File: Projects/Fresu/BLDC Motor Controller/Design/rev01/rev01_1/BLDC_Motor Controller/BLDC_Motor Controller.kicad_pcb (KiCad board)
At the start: 4 copper layers, 100 x 75 mm, 178 parts, among them CN1 XT60PW-M, J1 Conn_01x08, J2 Conn_01x06, J3 Conn_01x03, J4 7461084, J5 7461084, J6 7461084, J7 Conn_01x06, J8 XH-2PWBPZ, J9 TYPE-C-31-M-12, Q1 HSBA15810C, Q2 HSBA15810C, Q3 HSBA15810C, Q4 HSBA15810C, Q5 HSBA15810C, Q6 HSBA15810C, SW1 PTS526SK15SMTR2LFS, U1 STM32F405RGTx, U2 DRV8302_DCA_56, U3 S4B-XH-SM4-TB-(LF)(SN), U4 SN65HVD230, U5 AMS1117-3.3, U6 PUSB3AB6Z, Y1 8MHz

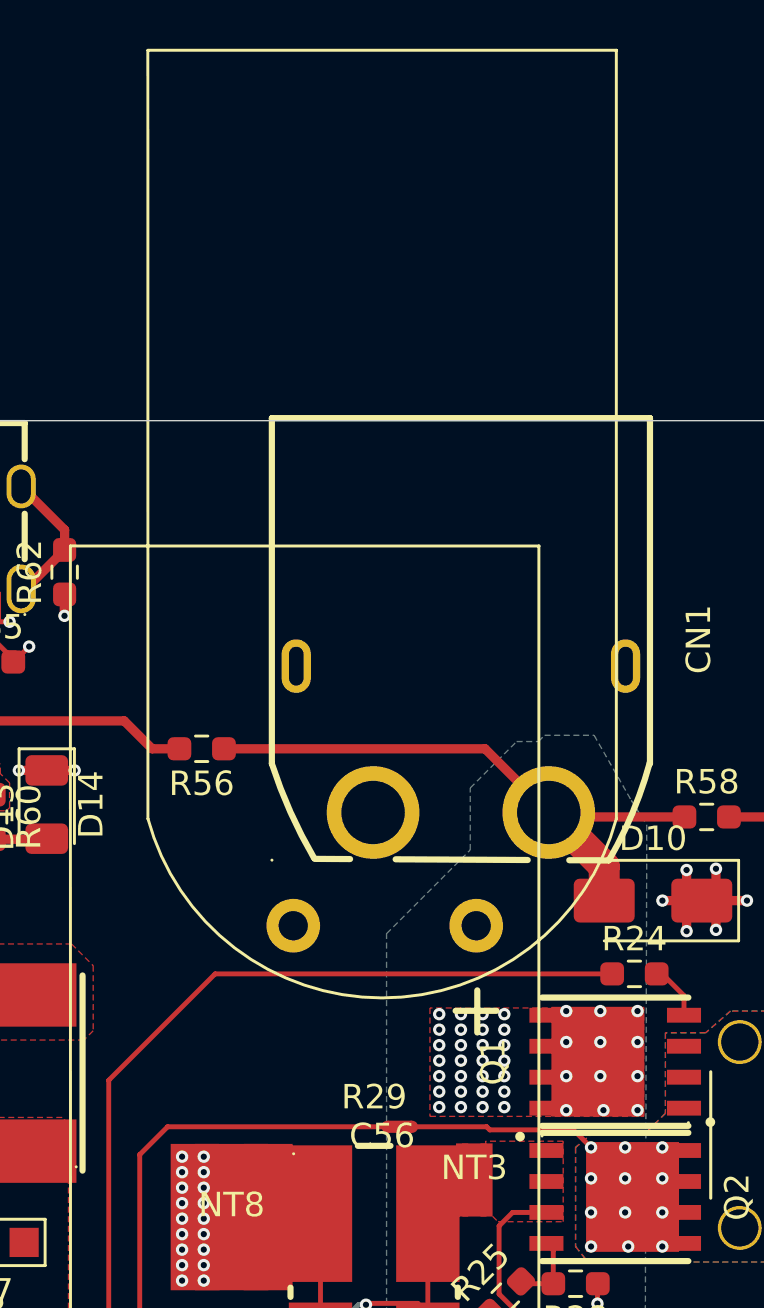
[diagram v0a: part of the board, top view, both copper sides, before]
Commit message: Update 22
Continued DRC
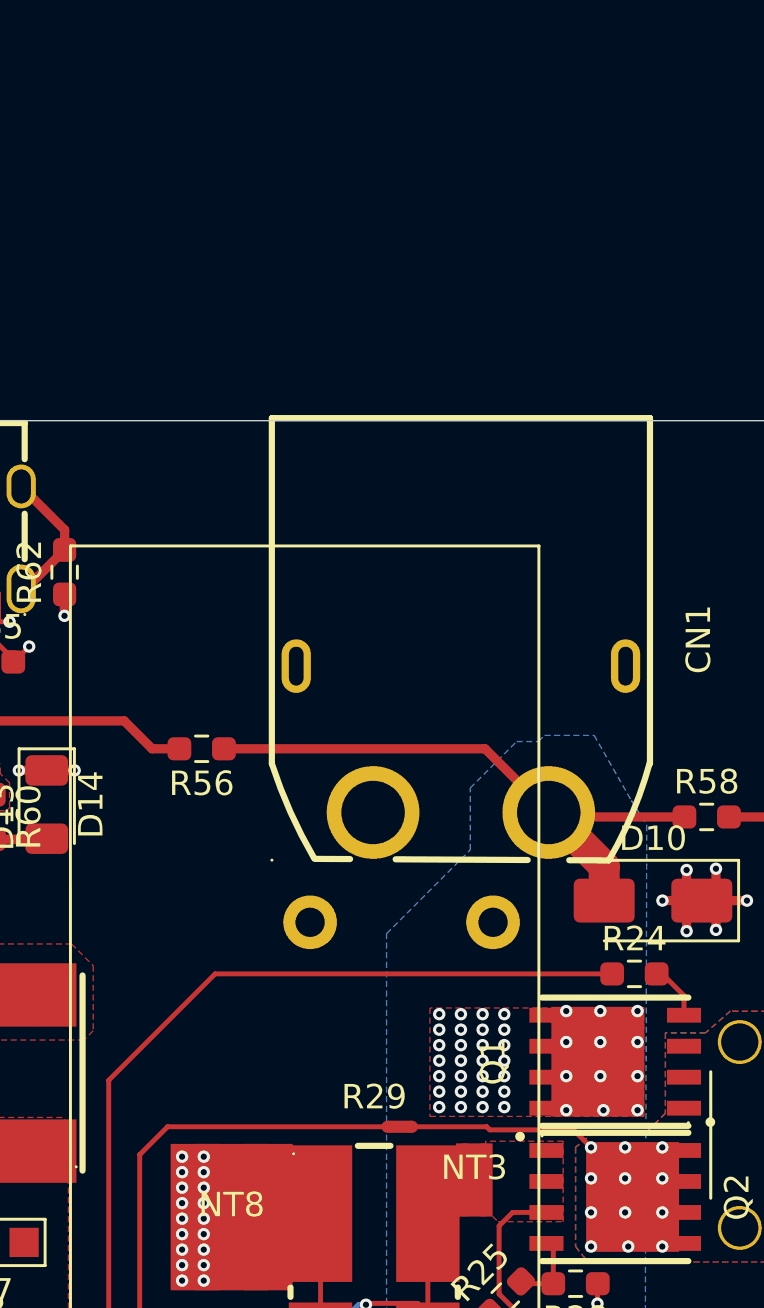
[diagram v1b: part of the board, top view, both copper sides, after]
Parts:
- C56: moved to B.Cu
- moved C56 0.78 mm to (238.6, 119.6)
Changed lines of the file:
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@@
     (pad "2" thru_hole circle locked (at 5.643701 0.113589 180) (size 2.2 2.2) (drill 1.2) (layers "*.Cu" "*.Mask")
       (net 2 "GND") (pinfunction "2") (pintype "passive"))
-    (model "C:/Users/Will/Downloads/Libraries (1)/Libraries/3D Models/CAP_LAT_SIDE.step"
+    (model "C:/Users/Will/Downloads/Libraries (1)/Libraries/3D Models/CAP_LAT_SIDE.step" hide
       (offset (xyz 1.9 -5.1 9.5))
       (scale (xyz 2.5 2.5 2.5))
@@
       (net 62 "H3_LOW") (pinfunction "2") (pintype "passive"))
   )
-  (footprint "DF_ESC_Footprint_Library:CAP-TH_BD18.0-P7.50-D1.2-SIDE" (layer "F.Cu")
-    (at 237.871 120.015 180)
-    (descr "CAP-TH_BD18.0-P7.50-D1.2-FD footprint")
-    (tags "CAP-TH_BD18.0-P7.50-D1.2-FD footprint")
-    (property "Capacitance" "820uF")
-    (property "LCSC" "C443097")
-    (property "Sheetfile" "INPUT PROTECTION.kicad_sch")
-    (property "Sheetname" "INPUT PROTECTION")
-    (property "ki_keywords" "C443097")
-    (attr through_hole)
-    (fp_text reference "C56" (at 2 -8.5) (layer "F.SilkS")
-        (effects (font (size 1 1) (thickness 0.15)))
-    )
-    (fp_text value "LKMI2501K821MF" (at 0 2.863602) (layer "F.Fab")
-        (effects (font (size 1 1) (thickness 0.15)))
-    )
-    (fp_text user "REF**" (at 0 4.863602) (layer "F.Fab")
-        (effects (font (size 1 1) (thickness 0.15)))
-    )
-    (fp_line (start -7.6 36) (end -7.6 4.5)
-      (stroke (width 0.12) (type solid)) (layer "F.SilkS"))
-    (fp_line (start -1.9 -2.536398) (end -1.9 -4.263602)
-      (stroke (width 0.254) (type solid)) (layer "F.SilkS"))
-    (fp_line (start -1.010998 -3.3746) (end -2.687402 -3.3746)
-      (stroke (width 0.254) (type solid)) (layer "F.SilkS"))
-    (fp_line (start 11.6 4.5) (end 11.604686 36)
-      (stroke (width 0.12) (type solid)) (layer "F.SilkS"))
-    (fp_line (start 11.6 36) (end -7.609372 36)
-      (stroke (width 0.12) (type solid)) (layer "F.SilkS"))
-    (fp_arc (start -7.6 4.5) (mid 2 -2.845853) (end 11.6 4.5)
-      (stroke (width 0.12) (type solid)) (layer "F.SilkS"))
-    (pad "1" thru_hole circle (at -1.856172 0.113589 180) (size 2.2 2.2) (drill 1.2) (layers "*.Cu" "*.Mask")
-      (net 18 "+VDC") (pinfunction "1") (pintype "passive"))
-    (pad "2" thru_hole circle (at 5.643701 0.113589 180) (size 2.2 2.2) (drill 1.2) (layers "*.Cu" "*.Mask")
-      (net 2 "GND") (pinfunction "2") (pintype "passive"))
-    (model "${DF_ESC_COURSE}/CAP_LAT_SIDE.step"
-      (offset (xyz 1.9 -5.1 9.5))
-      (scale (xyz 2.5 2.5 2.5))
-      (rotate (xyz -90 0 0))
-    )
-  )
   (footprint "DF_ESC_Footprint_Library:USB-C_SMD-TYPE-C-31-M-12" (layer "F.Cu")
     (at 216.748 103.08 180)
@@
     )
   )
+  (footprint "DF_ESC_Footprint_Library:CAP-TH_BD18.0-P7.50-D1.2-SIDE" (layer "B.Cu")
+    (at 238.561701 119.647411 180)
+    (descr "CAP-TH_BD18.0-P7.50-D1.2-FD footprint")
+    (tags "CAP-TH_BD18.0-P7.50-D1.2-FD footprint")
+    (property "Capacitance" "820uF")
+    (property "LCSC" "C443097")
+    (property "Sheetfile" "INPUT PROTECTION.kicad_sch")
+    (property "Sheetname" "INPUT PROTECTION")
+    (property "ki_keywords" "C443097")
+    (attr through_hole)
+    (fp_text reference "C56" (at 2 8.5) (layer "B.SilkS")
+        (effects (font (size 1 1) (thickness 0.15)) (justify mirror))
+    )
+    (fp_text value "LKMI2501K821MF" (at 0 -2.863602) (layer "B.Fab")
+        (effects (font (size 1 1) (thickness 0.15)) (justify mirror))
+    )
+    (fp_text user "REF**" (at 0 -4.863602) (layer "B.Fab")
+        (effects (font (size 1 1) (thickness 0.15)) (justify mirror))
+    )
+    (fp_line (start -7.6 -36) (end -7.6 -4.5)
+      (stroke (width 0.12) (type solid)) (layer "B.SilkS"))
+    (fp_line (start -1.9 2.536398) (end -1.9 4.263602)
+      (stroke (width 0.254) (type solid)) (layer "B.SilkS"))
+    (fp_line (start -1.010998 3.3746) (end -2.687402 3.3746)
+      (stroke (width 0.254) (type solid)) (layer "B.SilkS"))
+    (fp_line (start 11.6 -36) (end -7.609372 -36)
+      (stroke (width 0.12) (type solid)) (layer "B.SilkS"))
+    (fp_line (start 11.6 -4.5) (end 11.604686 -36)
+      (stroke (width 0.12) (type solid)) (layer "B.SilkS"))
+    (fp_arc (start 11.6 -4.5) (mid 2 2.845853) (end -7.6 -4.5)
+      (stroke (width 0.12) (type solid)) (layer "B.SilkS"))
+    (pad "1" thru_hole circle (at -1.856172 -0.113589 180) (size 2.2 2.2) (drill 1.2) (layers "*.Cu" "*.Mask")
+      (net 18 "+VDC") (pinfunction "1") (pintype "passive"))
+    (pad "2" thru_hole circle (at 5.643701 -0.113589 180) (size 2.2 2.2) (drill 1.2) (layers "*.Cu" "*.Mask")
+      (net 2 "GND") (pinfunction "2") (pintype "passive"))
+    (model "C:/Users/Will/Downloads/Libraries (1)/Libraries/3D Models/CAP_LAT_SIDE.step"
+      (offset (xyz 1.9 -5.1 9.5))
+      (scale (xyz 2.5 2.5 2.5))
+      (rotate (xyz -90 0 0))
+    )
+  )
